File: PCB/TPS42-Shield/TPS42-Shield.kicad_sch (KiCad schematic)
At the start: 26 parts, among them J1 PJ-320A, J10 FH12-10S-0.5SH, J11 Conn_01x06, J12 Conn_01x01, J2 Conn_01x06, J3 OLED, J4 PJ-320A, J5 Conn_01x06, J6 OLED, J7 FH12-10S-0.5SH, J8 Conn_01x06, J9 Conn_01x01

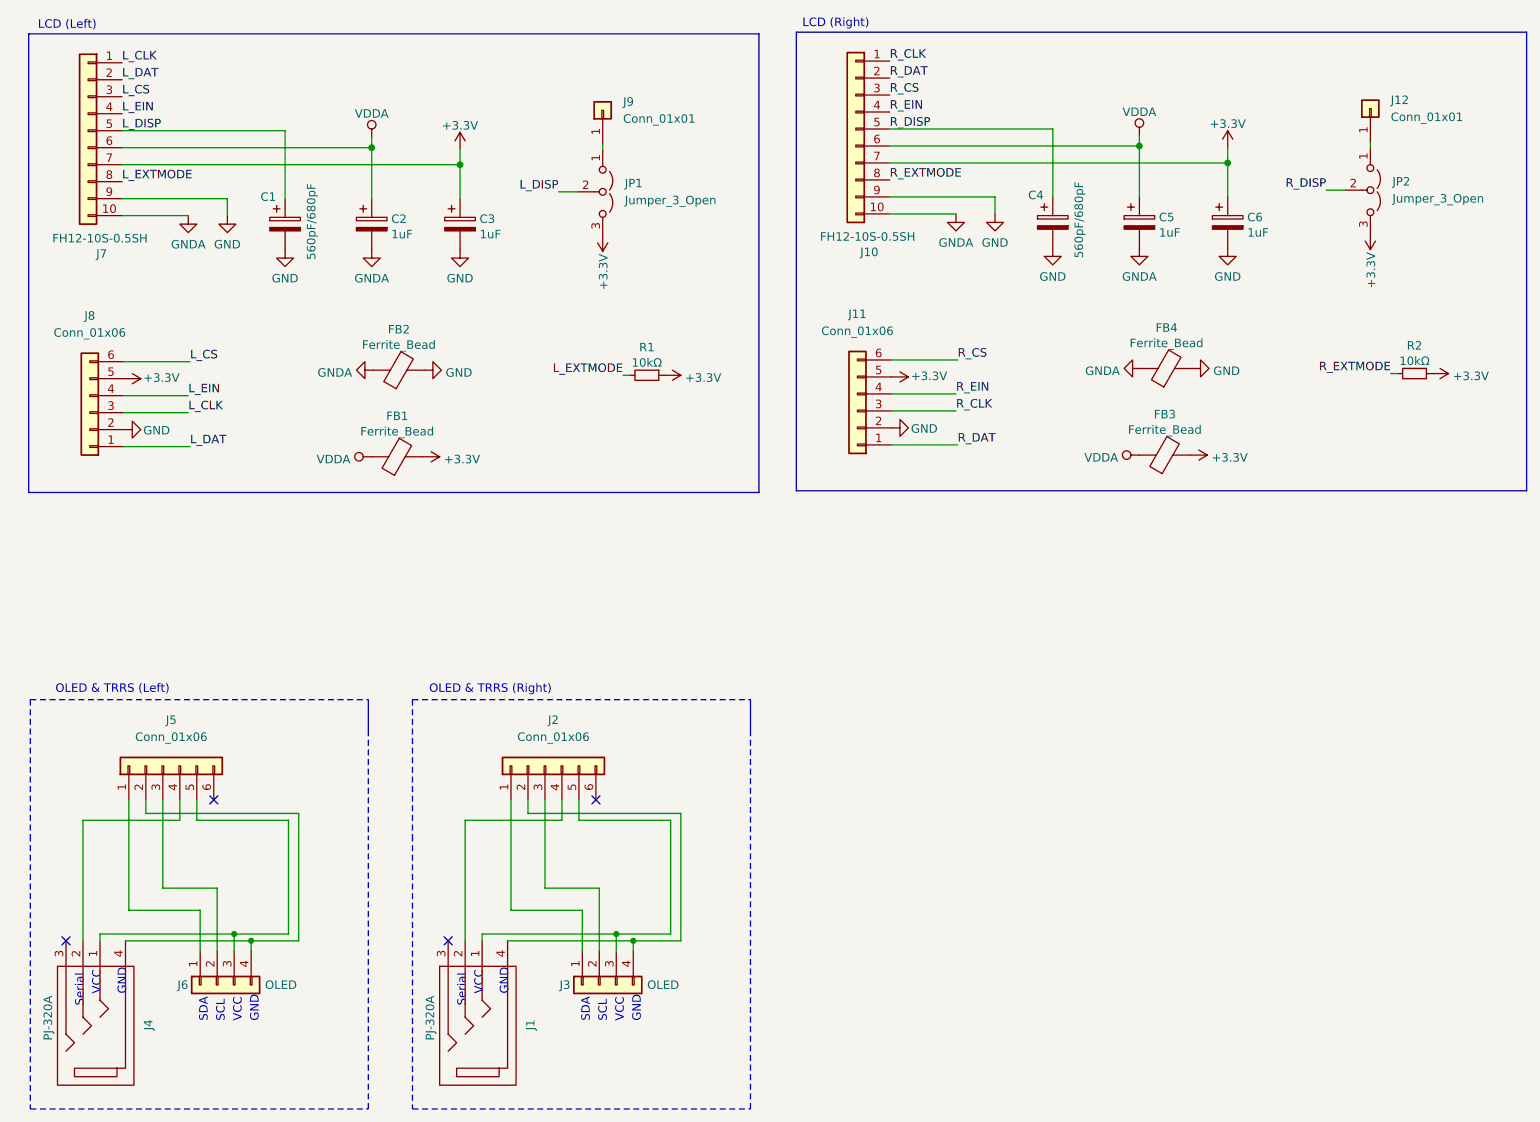
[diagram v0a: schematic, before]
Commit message: make it reversable (I)
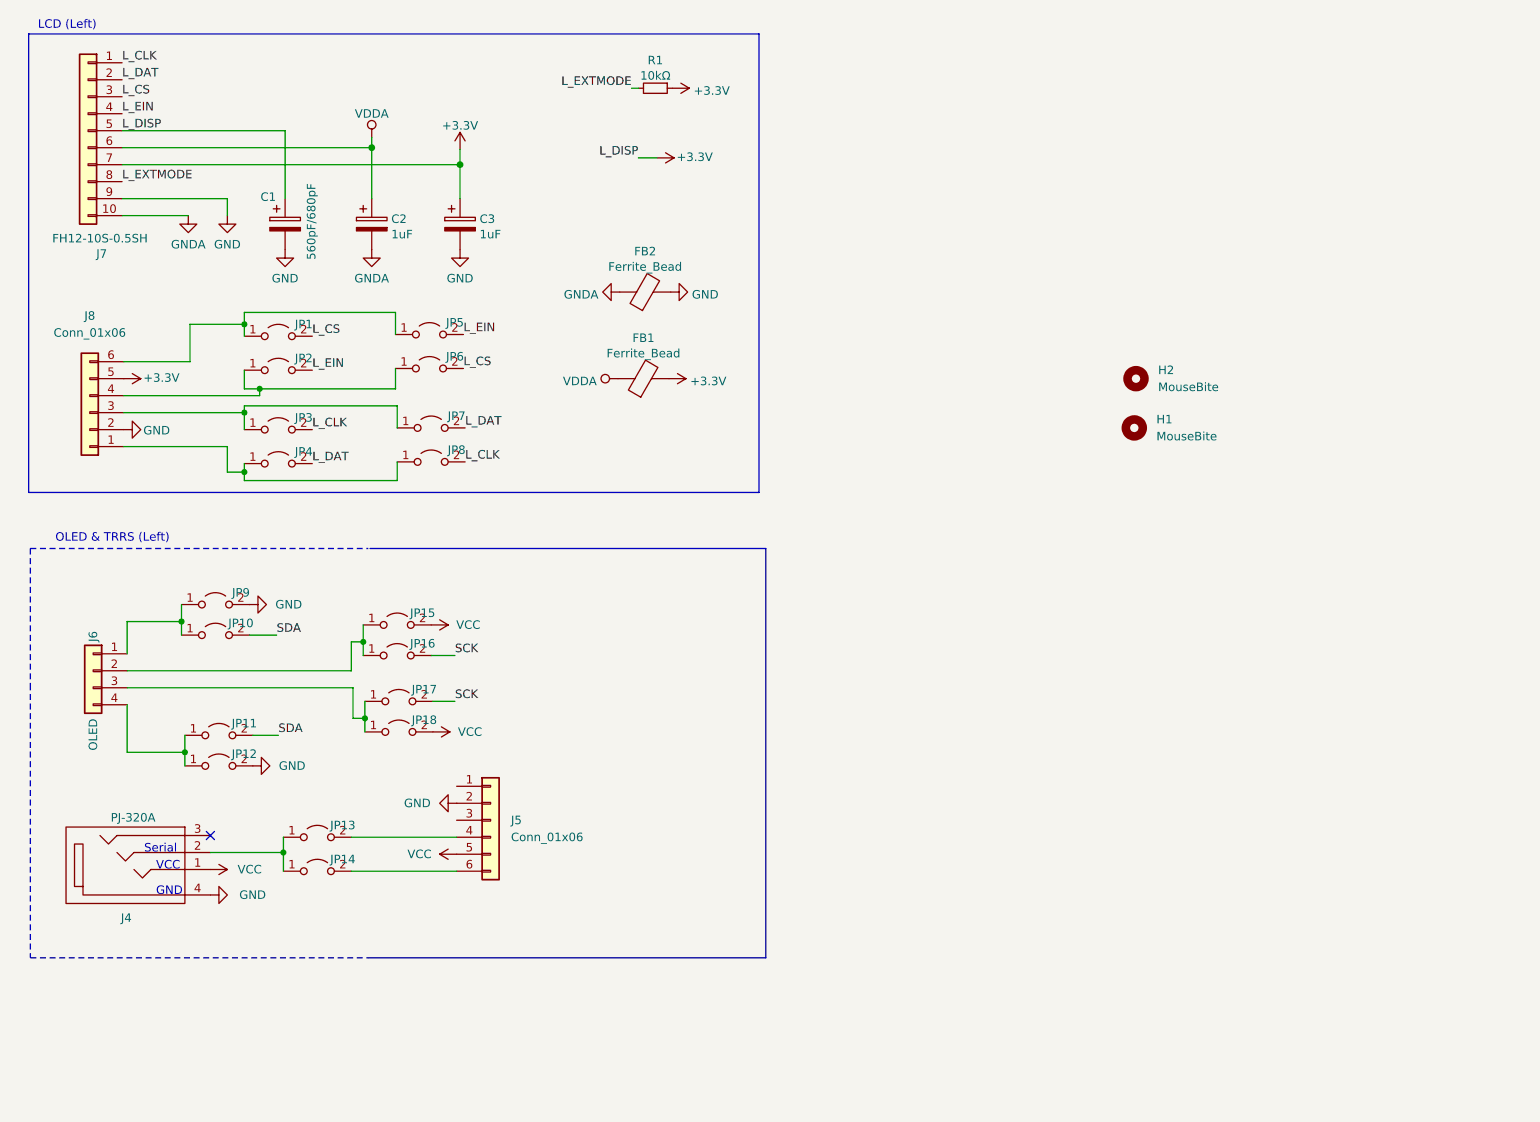
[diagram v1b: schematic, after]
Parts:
- removed C4: 560pF/680pF, Capacitor_SMD:C_0603_1608Metric_Pad1.08x0.95mm_HandSolder, symbol Device:CP
- removed C5, C6: 1uF, Capacitor_SMD:C_0603_1608Metric_Pad1.08x0.95mm_HandSolder, symbol Device:CP
- removed FB3, FB4: Ferrite_Bead, Resistor_SMD:R_0805_2012Metric_Pad1.20x1.40mm_HandSolder, symbol Device:Ferrite_Bead
- removed J1: PJ-320A, TPS42-Shield:MJ-4PP-9, symbol TPS42:MJ-4PP-9
- removed J10: FH12-10S-0.5SH, Connector_FFC-FPC:Hirose_FH12-10S-0.5SH_1x10-1MP_P0.50mm_Horizontal, symbol Connector_Generic:Conn_01x10
- removed J11, J2: Conn_01x06, Connector_PinHeader_2.54mm:PinHeader_2x03_P2.54mm_Vertical, symbol Connector_Generic:Conn_01x06
- removed J12, J9: Conn_01x01, Connector_PinHeader_2.54mm:PinHeader_1x01_P2.54mm_Vertical, symbol Connector_Generic:Conn_01x01
- removed J3: OLED, TPS42-Shield:OLED, symbol Connector_Generic:Conn_01x04
- removed JP1, JP2: Jumper_3_Open, Jumper:SolderJumper-3_P2.0mm_Open_TrianglePad1.0x1.5mm, symbol Jumper:Jumper_3_Open
- removed R2: 10kΩ, Resistor_SMD:R_0603_1608Metric_Pad0.98x0.95mm_HandSolder, symbol Device:R_Small
- added H1, H2: MouseBite, TPS42-Shield:mouse-bite-2mm-slot, symbol Mechanical:MountingHole
- added JP1, JP10, JP11, JP12, JP13, JP14, JP15, JP16, JP17, JP18, JP2, JP3, JP4, JP5, JP6, JP7, JP8, JP9: Jumper_2_Open, Jumper:SolderJumper-2_P1.3mm_Open_TrianglePad1.0x1.5mm, symbol Jumper:Jumper_2_Open
- J4: footprint TPS42-Shield:MJ-4PP-9 -> TPS42-Shield:MJ-4PP-9-reversable
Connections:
- net L_DISP is gone; now on net +3V3: C1.1, J7.5 (Pin_5)
- net GND: now also J4.4, J5.2 (Pin_2), JP12.2 (B), JP9.2 (B)
- net L_CLK: now also JP3.2 (B), JP8.2 (B); no longer J8.3 (Pin_3)
- net L_CS: now also JP1.2 (B), JP6.2 (B); no longer J8.6 (Pin_6)
- net L_DAT: now also JP4.2 (B), JP7.2 (B); no longer J8.1 (Pin_1)
- net L_EIN: now also JP2.2 (B), JP5.2 (B); no longer J8.4 (Pin_4)
- net at J6.1 (Pin_1): now also JP10.1 (A), JP9.1 (A); no longer J5.1 (Pin_1)
- net at J6.2 (Pin_2): now also JP15.1 (A), JP16.1 (A); no longer J5.3 (Pin_3)
- net VCC: now reaches J4.1, J5.5 (Pin_5)
- net VCC: now also JP15.2 (B), JP18.2 (B); no longer J6.3 (Pin_3)
- net at J4.2: now also JP13.1 (A), JP14.1 (A); no longer J5.4 (Pin_4)
- net at J5.6 (Pin_6): now also JP14.2 (B)
- new net: J6.3 (Pin_3), JP17.1 (A), JP18.1 (A)
- new net: J8.4 (Pin_4), JP2.1 (A), JP6.1 (A)
- new net: J6.4 (Pin_4), JP11.1 (A), JP12.1 (A)
- new net: J8.1 (Pin_1), JP4.1 (A), JP8.1 (A)
- new net: J8.3 (Pin_3), JP3.1 (A), JP7.1 (A)
- new net: J8.6 (Pin_6), JP1.1 (A), JP5.1 (A)
- new net: J5.4 (Pin_4), JP13.2 (B)
- new net SCK: JP16.2 (B), JP17.2 (B)
- new net SDA: JP10.2 (B), JP11.2 (B)
- no-connect marks 4 -> 1
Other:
- note removed: "LCD (Right)"
- note removed: "OLED & TRRS (Right)"
- note removed: "SCL"
- note removed: "SDA"
- moved on the sheet: FB1, FB2, J4, J5, J6, R1
